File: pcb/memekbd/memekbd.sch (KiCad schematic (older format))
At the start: 194 parts, among them J1 AudioJack4, J2 AudioJack4, SW1 SW_Push, SW10 SW_Push, SW11 SW_Push, SW12 SW_Push, SW13 SW_Push, SW14 SW_Push, SW15 SW_Push, SW16 SW_Push, SW17 SW_Push, SW18 SW_Push, SW19 SW_Push, SW2 SW_Push, SW20 SW_Push, SW21 SW_Push, SW22 SW_Push, SW23 SW_Push, SW24 SW_Push, SW25 SW_Push, SW26 SW_Push, SW27 SW_Push, SW28 SW_Push, SW29 SW_Push, SW3 SW_Push, SW30 SW_Push, SW31 SW_Push, SW32 SW_Push, SW33 SW_Push, SW34 SW_Push, SW35 SW_Push, SW36 SW_Push, SW37 SW_Push, SW38 SW_Push, SW39 SW_Push, SW4 SW_Push, SW40 SW_Push, SW41 SW_Push, SW42 SW_Push, SW43 SW_Push, SW44 SW_Push, SW45 SW_Push, SW46 SW_Push, SW47 SW_Push, SW48 SW_Push, SW5 SW_Push, SW6 SW_Push, SW7 SW_Push, SW8 SW_Push, SW9 SW_Push, U1 ProMicro, U2 ProMicro

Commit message: Assign footprints.
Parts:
- C1, C10, C11, C12, C13, C14, C15, C16, C17, C18, C19, C2, C20, C21, C22, C23, C24, C25, C26, C27, C28, C29, C3, C30, C31, C32, C33, C34, C35, C36, C37, C38, C39, C4, C40, C41, C42, C43, C44, C45, C46, C5, C6, C7, C8, C9: footprint (none) -> Capacitor_THT:C_Disc_D6.0mm_W2.5mm_P5.00mm
- J1, J2: footprint (none) -> kbd:MJ-4PP-9_1side
- LED1, LED10, LED11, LED12, LED13, LED14, LED15, LED16, LED17, LED18, LED19, LED2, LED20, LED21, LED22, LED23, LED24, LED25, LED26, LED27, LED28, LED29, LED3, LED30, LED31, LED32, LED33, LED34, LED35, LED36, LED37, LED38, LED39, LED4, LED40, LED41, LED42, LED43, LED44, LED45, LED46, LED5, LED6, LED7, LED8, LED9: footprint (none) -> kbd:YS-SK6812MINI-E
- R1, R2, R3, R4: footprint (none) -> Resistor_THT:R_Axial_DIN0207_L6.3mm_D2.5mm_P7.62mm_Horizontal
- SW1, SW10, SW11, SW12, SW13, SW14, SW15, SW16, SW17, SW18, SW19, SW2, SW20, SW21, SW22, SW23, SW24, SW25, SW26, SW27, SW28, SW29, SW3, SW30, SW31, SW32, SW33, SW34, SW35, SW36, SW37, SW38, SW39, SW4, SW40, SW41, SW42, SW43, SW44, SW45, SW46, SW5, SW6, SW7, SW8, SW9: footprint (none) -> kbd:CherryMX_Hotswap
- SW47, SW48: footprint (none) -> Button_Switch_THT:SW_PUSH_6mm_H7.3mm
- U1, U2: footprint (none) -> kbd:ProMicro_v3.5

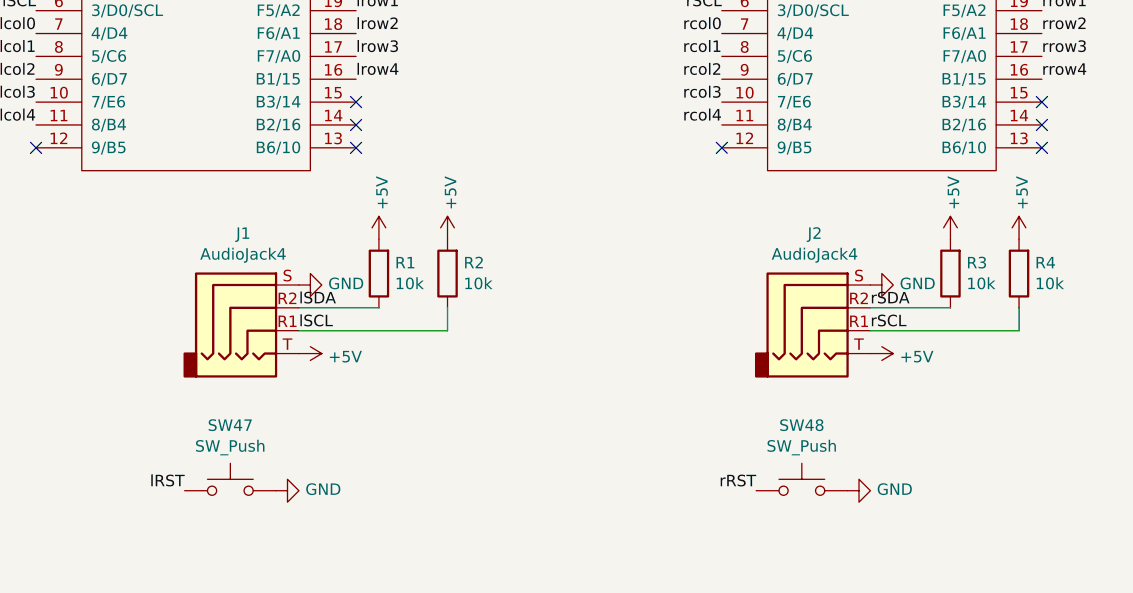
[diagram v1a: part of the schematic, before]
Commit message: Most of pcb layout work.
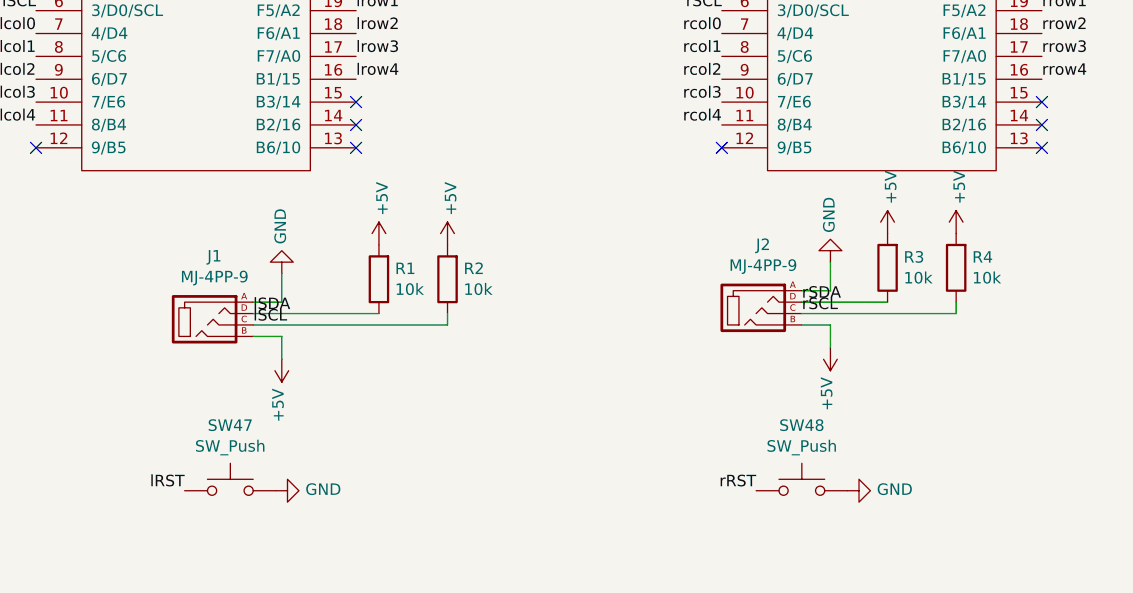
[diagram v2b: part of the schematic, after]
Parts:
- removed J1, J2: AudioJack4, kbd:MJ-4PP-9_1side, symbol Connector:AudioJack4
- added J1, J2: MJ-4PP-9, kbd:MJ-4PP-9_1side, symbol kbd:MJ-4PP-9
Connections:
- net +5V: now also J1.B, J2.B
- net GND: now also J1.A, J2.A
- net lSCL: now also J1.C
- net lSDA: now also J1.D
- net rSCL: now also J2.C
- net rSDA: now also J2.D
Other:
- moved on the sheet: R1, R2, R3, R4
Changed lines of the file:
@@
 $EndComp
 $Comp
-L Connector:AudioJack4 J1
-U 1 1 60D94451
-P 15750 3650
-F 0 "J1" H 15707 3975 50  0000 C CNN
-F 1 "AudioJack4" H 15707 3884 50  0000 C CNN
-F 2 "kbd:MJ-4PP-9_1side" H 15750 3650 50  0001 C CNN
-F 3 "~" H 15750 3650 50  0001 C CNN
-	1    15750 3650
-	1    0    0    -1
-$EndComp
-$Comp
-L Connector:AudioJack4 J2
-U 1 1 60D97F5C
-P 18250 3650
-F 0 "J2" H 18207 3975 50  0000 C CNN
-F 1 "AudioJack4" H 18207 3884 50  0000 C CNN
-F 2 "kbd:MJ-4PP-9_1side" H 18250 3650 50  0001 C CNN
-F 3 "~" H 18250 3650 50  0001 C CNN
-	1    18250 3650
-	1    0    0    -1
-$EndComp
-$Comp
 L power:GND #PWR0129
 U 1 1 60D9B008
@@
 L power:GND #PWR0127
 U 1 1 60D9B386
-P 15950 3550
-F 0 "#PWR0127" H 15950 3300 50  0001 C CNN
-F 1 "GND" V 15955 3422 50  0000 R CNN
-F 2 "" H 15950 3550 50  0001 C CNN
-F 3 "" H 15950 3550 50  0001 C CNN
-	1    15950 3550
-	0    -1   -1   0
-$EndComp
-$Comp
-L power:GND #PWR0136
-U 1 1 60D9B90C
-P 18450 3550
-F 0 "#PWR0136" H 18450 3300 50  0001 C CNN
-F 1 "GND" V 18455 3422 50  0000 R CNN
-F 2 "" H 18450 3550 50  0001 C CNN
-F 3 "" H 18450 3550 50  0001 C CNN
-	1    18450 3550
-	0    -1   -1   0
+P 15875 3500
+F 0 "#PWR0127" H 15875 3250 50  0001 C CNN
+F 1 "GND" V 15880 3372 50  0000 R CNN
+F 2 "" H 15875 3500 50  0001 C CNN
+F 3 "" H 15875 3500 50  0001 C CNN
+	1    15875 3500
+	-1   0    0    1
 $EndComp
 $Comp
@@
 L power:+5V #PWR0128
 U 1 1 60D9D453
-P 15950 3850
-F 0 "#PWR0128" H 15950 3700 50  0001 C CNN
-F 1 "+5V" V 15965 3978 50  0000 L CNN
-F 2 "" H 15950 3850 50  0001 C CNN
-F 3 "" H 15950 3850 50  0001 C CNN
-	1    15950 3850
-	0    1    1    0
-$EndComp
-$Comp
-L power:+5V #PWR0137
-U 1 1 60D9DA3D
-P 18450 3850
-F 0 "#PWR0137" H 18450 3700 50  0001 C CNN
-F 1 "+5V" V 18465 3978 50  0000 L CNN
-F 2 "" H 18450 3850 50  0001 C CNN
-F 3 "" H 18450 3850 50  0001 C CNN
-	1    18450 3850
-	0    1    1    0
+P 15875 3875
+F 0 "#PWR0128" H 15875 3725 50  0001 C CNN
+F 1 "+5V" V 15890 4003 50  0000 L CNN
+F 2 "" H 15875 3875 50  0001 C CNN
+F 3 "" H 15875 3875 50  0001 C CNN
+	1    15875 3875
+	-1   0    0    1
 $EndComp
 $Comp
@@
 lSCL
 $Comp
-L Device:R R1
-U 1 1 60DFBED0
-P 16300 3500
-F 0 "R1" H 16230 3454 50  0000 R CNN
-F 1 "10k" H 16230 3545 50  0000 R CNN
-F 2 "Resistor_THT:R_Axial_DIN0207_L6.3mm_D2.5mm_P7.62mm_Horizontal" V 16230 3500 50  0001 C CNN
-F 3 "~" H 16300 3500 50  0001 C CNN
-	1    16300 3500
-	-1   0    0    1
-$EndComp
-$Comp
-L power:+5V #PWR0131
-U 1 1 60DFD705
-P 16300 3350
-F 0 "#PWR0131" H 16300 3200 50  0001 C CNN
-F 1 "+5V" V 16315 3478 50  0000 L CNN
-F 2 "" H 16300 3350 50  0001 C CNN
-F 3 "" H 16300 3350 50  0001 C CNN
-	1    16300 3350
-	1    0    0    -1
-$EndComp
-$Comp
 L Device:R R2
 U 1 1 60E00297
-P 16600 3500
-F 0 "R2" H 16530 3454 50  0000 R CNN
-F 1 "10k" H 16530 3545 50  0000 R CNN
-F 2 "Resistor_THT:R_Axial_DIN0207_L6.3mm_D2.5mm_P7.62mm_Horizontal" V 16530 3500 50  0001 C CNN
-F 3 "~" H 16600 3500 50  0001 C CNN
-	1    16600 3500
+P 16600 3525
+F 0 "R2" H 16530 3479 50  0000 R CNN
+F 1 "10k" H 16530 3570 50  0000 R CNN
+F 2 "Resistor_THT:R_Axial_DIN0207_L6.3mm_D2.5mm_P7.62mm_Horizontal" V 16530 3525 50  0001 C CNN
+F 3 "~" H 16600 3525 50  0001 C CNN
+	1    16600 3525
 	-1   0    0    1
 $EndComp
@@
 L power:+5V #PWR0132
 U 1 1 60E0029D
-P 16600 3350
-F 0 "#PWR0132" H 16600 3200 50  0001 C CNN
-F 1 "+5V" V 16615 3478 50  0000 L CNN
-F 2 "" H 16600 3350 50  0001 C CNN
-F 3 "" H 16600 3350 50  0001 C CNN
-	1    16600 3350
+P 16600 3375
+F 0 "#PWR0132" H 16600 3225 50  0001 C CNN
+F 1 "+5V" V 16615 3503 50  0000 L CNN
+F 2 "" H 16600 3375 50  0001 C CNN
+F 3 "" H 16600 3375 50  0001 C CNN
+	1    16600 3375
 	1    0    0    -1
 $EndComp
 Wire Wire Line
-	16600 3750 16600 3650
+	16600 3725 16600 3675
 Wire Wire Line
-	15950 3750 16600 3750
-Wire Wire Line
-	15950 3650 16300 3650
-Text Label 15950 3650 0    50   ~ 0
+	15750 3725 16600 3725
+Text Label 15750 3675 0    50   ~ 0
 lSDA
-Text Label 15950 3750 0    50   ~ 0
+Text Label 15750 3725 0    50   ~ 0
 lSCL
 Text Label 17800 2250 2    50   ~ 0
@@
 L Device:R R3
 U 1 1 60E5D7AF
-P 18800 3500
-F 0 "R3" H 18730 3454 50  0000 R CNN
-F 1 "10k" H 18730 3545 50  0000 R CNN
-F 2 "Resistor_THT:R_Axial_DIN0207_L6.3mm_D2.5mm_P7.62mm_Horizontal" V 18730 3500 50  0001 C CNN
-F 3 "~" H 18800 3500 50  0001 C CNN
-	1    18800 3500
+P 18525 3475
+F 0 "R3" H 18455 3429 50  0000 R CNN
+F 1 "10k" H 18455 3520 50  0000 R CNN
+F 2 "Resistor_THT:R_Axial_DIN0207_L6.3mm_D2.5mm_P7.62mm_Horizontal" V 18455 3475 50  0001 C CNN
+F 3 "~" H 18525 3475 50  0001 C CNN
+	1    18525 3475
 	-1   0    0    1
 $EndComp
@@
 L power:+5V #PWR0138
 U 1 1 60E5D7B5
-P 18800 3350
-F 0 "#PWR0138" H 18800 3200 50  0001 C CNN
-F 1 "+5V" V 18815 3478 50  0000 L CNN
-F 2 "" H 18800 3350 50  0001 C CNN
-F 3 "" H 18800 3350 50  0001 C CNN
-	1    18800 3350
+P 18525 3325
+F 0 "#PWR0138" H 18525 3175 50  0001 C CNN
+F 1 "+5V" V 18540 3453 50  0000 L CNN
+F 2 "" H 18525 3325 50  0001 C CNN
+F 3 "" H 18525 3325 50  0001 C CNN
+	1    18525 3325
 	1    0    0    -1
 $EndComp
@@
 L Device:R R4
 U 1 1 60E5D7BB
-P 19100 3500
-F 0 "R4" H 19030 3454 50  0000 R CNN
-F 1 "10k" H 19030 3545 50  0000 R CNN
-F 2 "Resistor_THT:R_Axial_DIN0207_L6.3mm_D2.5mm_P7.62mm_Horizontal" V 19030 3500 50  0001 C CNN
-F 3 "~" H 19100 3500 50  0001 C CNN
-	1    19100 3500
+P 18825 3475
+F 0 "R4" H 18755 3429 50  0000 R CNN
+F 1 "10k" H 18755 3520 50  0000 R CNN
+F 2 "Resistor_THT:R_Axial_DIN0207_L6.3mm_D2.5mm_P7.62mm_Horizontal" V 18755 3475 50  0001 C CNN
+F 3 "~" H 18825 3475 50  0001 C CNN
+	1    18825 3475
 	-1   0    0    1
 $EndComp
@@
 L power:+5V #PWR0139
 U 1 1 60E5D7C1
-P 19100 3350
-F 0 "#PWR0139" H 19100 3200 50  0001 C CNN
-F 1 "+5V" V 19115 3478 50  0000 L CNN
-F 2 "" H 19100 3350 50  0001 C CNN
-F 3 "" H 19100 3350 50  0001 C CNN
-	1    19100 3350
+P 18825 3325
+F 0 "#PWR0139" H 18825 3175 50  0001 C CNN
+F 1 "+5V" V 18840 3453 50  0000 L CNN
+F 2 "" H 18825 3325 50  0001 C CNN
+F 3 "" H 18825 3325 50  0001 C CNN
+	1    18825 3325
 	1    0    0    -1
 $EndComp
 Wire Wire Line
-	19100 3750 19100 3650
+	18825 3675 18825 3625
 Wire Wire Line
-	18450 3750 19100 3750
+	18150 3675 18825 3675
 Wire Wire Line
-	18450 3650 18800 3650
-Text Label 18450 3650 0    50   ~ 0
+	18150 3625 18525 3625
+Text Label 18150 3625 0    50   ~ 0
 rSDA
-Text Label 18450 3750 0    50   ~ 0
+Text Label 18150 3675 0    50   ~ 0
 rSCL
 Text Label 2100 7000 2    50   ~ 0
@@
 $EndComp
 NoConn ~ 19200 1850
+$Comp
+L kbd:MJ-4PP-9 J1
+U 1 1 614F36EF
+P 15550 3700
+F 0 "J1" H 15581 3976 50  0000 C CNN
+F 1 "MJ-4PP-9" H 15581 3885 50  0000 C CNN
+F 2 "kbd:MJ-4PP-9_1side" H 15825 3875 50  0001 C CNN
+F 3 "~" H 15825 3875 50  0001 C CNN
+	1    15550 3700
+	1    0    0    -1
+$EndComp
+$Comp
+L kbd:MJ-4PP-9 J2
+U 1 1 614F5099
+P 17950 3650
+F 0 "J2" H 17981 3926 50  0000 C CNN
+F 1 "MJ-4PP-9" H 17981 3835 50  0000 C CNN
+F 2 "kbd:MJ-4PP-9_1side" H 18225 3825 50  0001 C CNN
+F 3 "~" H 18225 3825 50  0001 C CNN
+	1    17950 3650
+	1    0    0    -1
+$EndComp
+Wire Wire Line
+	15750 3625 15875 3625
+Wire Wire Line
+	15875 3625 15875 3500
+Wire Wire Line
+	15750 3775 15875 3775
+Wire Wire Line
+	15875 3775 15875 3875
+Wire Wire Line
+	15750 3675 16300 3675
+$Comp
+L power:+5V #PWR0131
+U 1 1 60DFD705
+P 16300 3375
+F 0 "#PWR0131" H 16300 3225 50  0001 C CNN
+F 1 "+5V" V 16315 3503 50  0000 L CNN
+F 2 "" H 16300 3375 50  0001 C CNN
+F 3 "" H 16300 3375 50  0001 C CNN
+	1    16300 3375
+	1    0    0    -1
+$EndComp
+$Comp
+L Device:R R1
+U 1 1 60DFBED0
+P 16300 3525
+F 0 "R1" H 16230 3479 50  0000 R CNN
+F 1 "10k" H 16230 3570 50  0000 R CNN
+F 2 "Resistor_THT:R_Axial_DIN0207_L6.3mm_D2.5mm_P7.62mm_Horizontal" V 16230 3525 50  0001 C CNN
+F 3 "~" H 16300 3525 50  0001 C CNN
+	1    16300 3525
+	-1   0    0    1
+$EndComp
+$Comp
+L power:+5V #PWR0136
+U 1 1 615CFE82
+P 18275 3825
+F 0 "#PWR0136" H 18275 3675 50  0001 C CNN
+F 1 "+5V" V 18290 3953 50  0000 L CNN
+F 2 "" H 18275 3825 50  0001 C CNN
+F 3 "" H 18275 3825 50  0001 C CNN
+	1    18275 3825
+	-1   0    0    1
+$EndComp
+Wire Wire Line
+	18150 3725 18275 3725
+Wire Wire Line
+	18275 3725 18275 3825
+$Comp
+L power:GND #PWR0137
+U 1 1 615D8D20
+P 18275 3450
+F 0 "#PWR0137" H 18275 3200 50  0001 C CNN
+F 1 "GND" V 18280 3322 50  0000 R CNN
+F 2 "" H 18275 3450 50  0001 C CNN
+F 3 "" H 18275 3450 50  0001 C CNN
+	1    18275 3450
+	-1   0    0    1
+$EndComp
+Wire Wire Line
+	18275 3575 18275 3450
+Wire Wire Line
+	18275 3575 18150 3575
 $EndSCHEMATC
